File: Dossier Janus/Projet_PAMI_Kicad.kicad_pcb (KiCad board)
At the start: 4 copper layers, 61 x 38.5 mm, 35 parts, among them J1 FTSH-107-01-F-DV-K, U11 STM32L552CCTx, U12 R-78B5.0-2.0, U7 AZ1117-3.3, U9 TB6612FNG

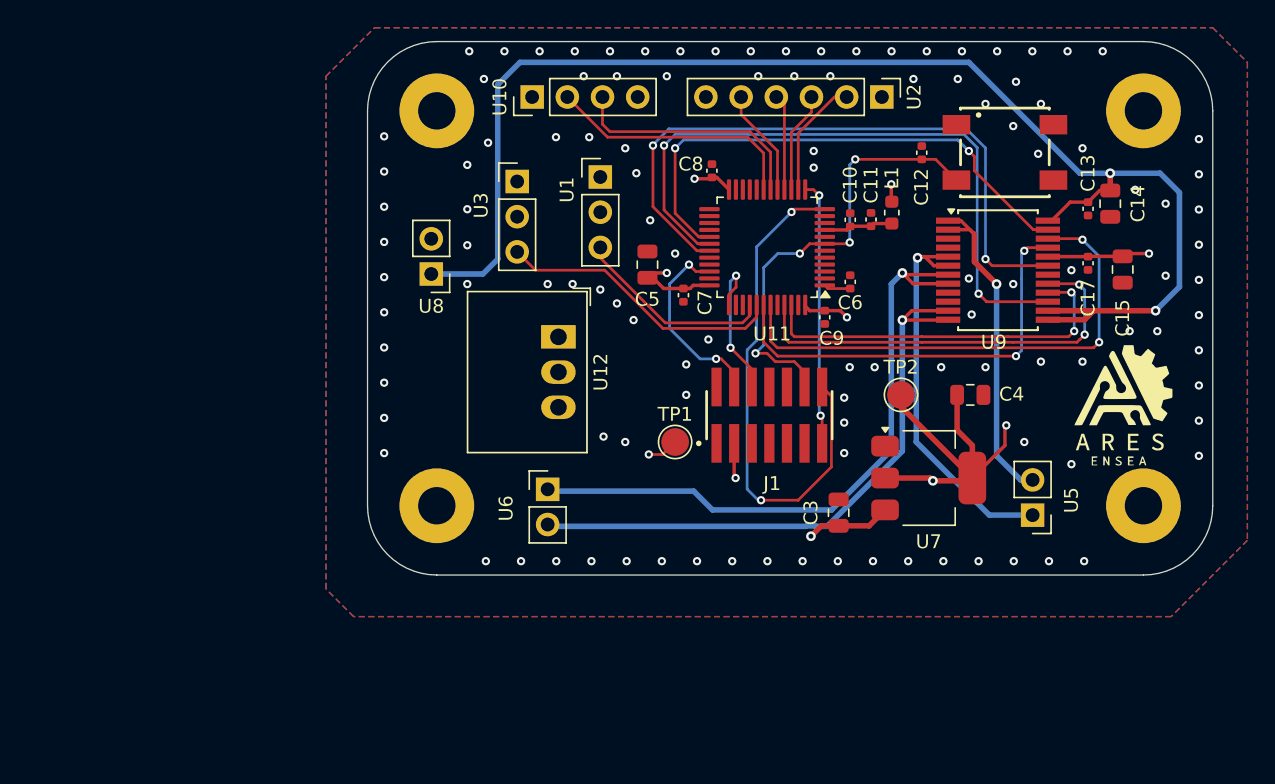
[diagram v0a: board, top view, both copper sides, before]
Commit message: Finalisation du PCB--Dossier Janus
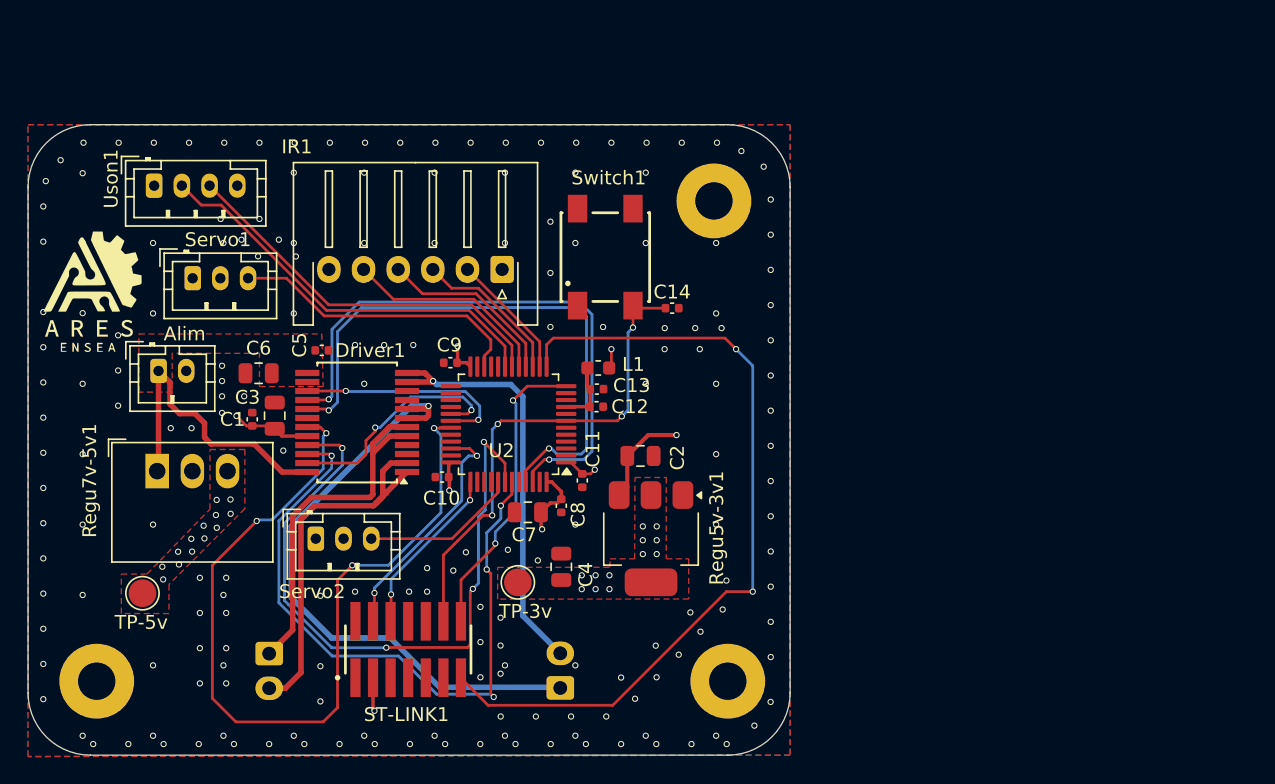
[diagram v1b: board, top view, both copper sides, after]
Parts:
- removed C15: 10u, Capacitor_SMD:C_0805_2012Metric
- removed C17: 100n, Capacitor_SMD:C_0402_1005Metric
- removed H4: MountingHole_Pad, MountingHole:MountingHole_2.7mm_M2.5_Pad
- removed J1: FTSH-107-01-F-DV-K, FTSH-107-01-F-DV-K:SAMTEC_FTSH-107-01-F-DV-K
- removed S1: 430471025826, boutonSMD_wurth430471025826:430471025826
- removed TP1, TP2: TestPoint, TestPoint:TestPoint_Pad_D2.0mm
- removed U1, U3: ~, Connector_PinHeader_2.54mm:PinHeader_1x03_P2.54mm_Vertical
- removed U10: ~, Connector_PinHeader_2.54mm:PinHeader_1x04_P2.54mm_Vertical
- removed U11: STM32L552CCTx, Package_QFP:LQFP-48_7x7mm_P0.5mm
- removed U12: R-78B5.0-2.0, Converter_DCDC:Converter_DCDC_RECOM_R-78B-2.0_THT
- removed U5, U6, U8: ~, Connector_PinHeader_2.54mm:PinHeader_1x02_P2.54mm_Vertical
- removed U7: AZ1117-3.3, Package_TO_SOT_SMD:SOT-223-3_TabPin2
- removed U9: TB6612FNG, Package_SO:SSOP-24_5.3x8.2mm_P0.65mm
- added Alim: ~, Connector_JST:JST_PH_B2B-PH-K_1x02_P2.00mm_Vertical, F.Cu at (96.9, 75.3)
- added C1: 100n, Capacitor_SMD:C_0402_1005Metric, F.Cu at (103.7, 78.8)
- added C2: 10u, Capacitor_SMD:C_0805_2012Metric, F.Cu at (131.7, 81.4)
- added Driver1: TB6612FNG, Package_SO:SSOP-24_5.3x8.2mm_P0.65mm, F.Cu at (111.3, 79.0)
- added IR1: ~, Connector_JST:JST_XH_S6B-XH-A-1_1x06_P2.50mm_Horizontal, F.Cu at (121.7, 67.9)
- added Moteur1: ~, Connector_JST:JST_XH_B2B-XH-A_1x02_P2.50mm_Vertical, B.Cu at (104.9, 95.7)
- added Moteur2: ~, Connector_JST:JST_XH_B2B-XH-A_1x02_P2.50mm_Vertical, B.Cu at (125.9, 98.2)
- added Regu5v-3v1: AZ1117-3.3, Package_TO_SOT_SMD:SOT-223-3_TabPin2, F.Cu at (132.5, 87.4)
- added Regu7v-5v1: R-78B5.0-2.0, Converter_DCDC:Converter_DCDC_RECOM_R-78B-2.0_THT, F.Cu at (96.8, 82.5)
- added ST-LINK1: FTSH-107-01-F-DV-K, FTSH-107-01-F-DV-K:SAMTEC_FTSH-107-01-F-DV-K, F.Cu at (114.9, 95.4)
- added Servo1: ~, Connector_JST:JST_PH_B3B-PH-K_1x03_P2.00mm_Vertical, F.Cu at (99.4, 68.6)
- added Servo2: ~, Connector_JST:JST_PH_B3B-PH-K_1x03_P2.00mm_Vertical, F.Cu at (108.3, 87.4)
- added Switch1: 430471025826, boutonSMD_wurth430471025826:430471025826, F.Cu at (129.2, 67.1)
- added TP-3v: TestPoint, TestPoint:TestPoint_Pad_D2.0mm, F.Cu at (122.8, 90.5)
- added TP-5v: TestPoint, TestPoint:TestPoint_Pad_D2.0mm, F.Cu at (95.8, 91.3)
- added Uson1: ~, Connector_JST:JST_PH_B4B-PH-K_1x04_P2.00mm_Vertical, F.Cu at (96.6, 61.9)
- C10: value 10n -> 100n
- C11: value 1u -> 100n
- C13: value 100n -> 1u
- C14: value 10u -> 10n; footprint Capacitor_SMD:C_0805_2012Metric -> Capacitor_SMD:C_0402_1005Metric
- C5: value 4u7 -> 100n; footprint Capacitor_SMD:C_0805_2012Metric -> Capacitor_SMD:C_0402_1005Metric
- C6: value 100n -> 10u; footprint Capacitor_SMD:C_0402_1005Metric -> Capacitor_SMD:C_0805_2012Metric
- C7: value 100n -> 4u7; footprint Capacitor_SMD:C_0402_1005Metric -> Capacitor_SMD:C_0805_2012Metric
- U2: value ~ -> MCU; footprint Connector_PinHeader_2.54mm:PinHeader_1x06_P2.54mm_Vertical -> Package_QFP:LQFP-48_7x7mm_P0.5mm
- moved G*** 74.9 mm to (92.0, 69.8)
- moved H1 47.9 mm to (92.5, 97.7)
- moved C6 43.2 mm to (104.1, 75.4), turned to 180 degrees
- moved C3 41.3 mm to (105.3, 78.5)
- moved C13 37.8 mm to (128.6, 76.6), turned to 0 degrees
- moved U2 35.8 mm to (122.2, 79.1), turned to 180 degrees
- moved C10 34.8 mm to (117.4, 82.9), turned to 180 degrees
- moved H3 32.6 mm to (138.0, 97.7)
- moved C14 32.5 mm to (134.0, 70.7), turned to 0 degrees
- moved C4 32.0 mm to (126.0, 89.4), turned to 90 degrees
- moved H2 31.7 mm to (137.0, 63.0)
- moved C12 29.8 mm to (128.5, 77.9), turned to 0 degrees
- moved C11 28.1 mm to (127.5, 83.2), turned to -90 degrees
- moved C9 27.2 mm to (118.0, 74.7), turned to 180 degrees
- moved C8 26.5 mm to (126.0, 85.0), turned to -90 degrees
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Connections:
- C10 pad 1: +3.3VA -> +3.3V
- C11 pad 1: +3.3VA -> +3.3V
- C12 pad 1: /NRST -> +3.3VA
- C13 pad 1: +7.5V -> +3.3VA
- C14 pad 1: +7.5V -> /NRST
- C3 pad 1: +5V -> +3.3V
- C5 pad 1: +3.3V -> +7.5V
- C6 pad 1: +3.3V -> +7.5V
- U2 pad 1: +5V -> +3.3V
- U2 pad 2: /IR_1 -> unconnected-(U2-PC13-Pad2)
- U2 pad 3: /IR_2 -> unconnected-(U2-PC14-Pad3)
- U2 pad 4: /IR_3 -> unconnected-(U2-PC15-Pad4)
- U2 pad 5: /IR_4 -> unconnected-(U2-PH0-Pad5)
- U2 pad 6: GND -> unconnected-(U2-PH1-Pad6)
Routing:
- net +7.5V: track 98.8 -> 22.6 mm, vias 2 -> 0
- net /STLINK_RX: track 20.3 -> 59.1 mm
- net /PWMB: track 48.1 -> 16.0 mm
- net +3.3V: track 51.5 -> 21.5 mm, vias 8 -> 19
- net /PWMA: track 38.3 -> 16.8 mm
- net /AIN1: track 31.0 -> 48.9 mm, vias 2 -> 4
- net /STLINK_TX: track 37.3 -> 21.9 mm
- net /BIN2: track 27.3 -> 42.2 mm
- net /BO1: track 44.3 -> 30.6 mm
- net /STBY: track 47.6 -> 61.1 mm, vias 2 -> 4
- net /BIN1: track 30.5 -> 42.2 mm
- net /AIN2: track 37.1 -> 48.8 mm, vias 2 -> 4
- net /Trig: track 18.5 -> 29.6 mm
- net /Echo: track 17.6 -> 28.1 mm
- net /PWM_Servo2: track 20.8 -> 11.3 mm
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- added copper zone on F.Cu, net +3.3V
- added copper zone on F.Cu, net +5V
- added copper zone on F.Cu, net +7.5V
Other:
- board size 61 x 38.5 mm -> 55 x 45.5 mm
- board text removed: "PROJET PAMI ARES 1A"
